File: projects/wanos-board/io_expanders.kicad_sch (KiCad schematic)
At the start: 17 parts, among them U1 PCA9554PW, U2 PCA9554PW

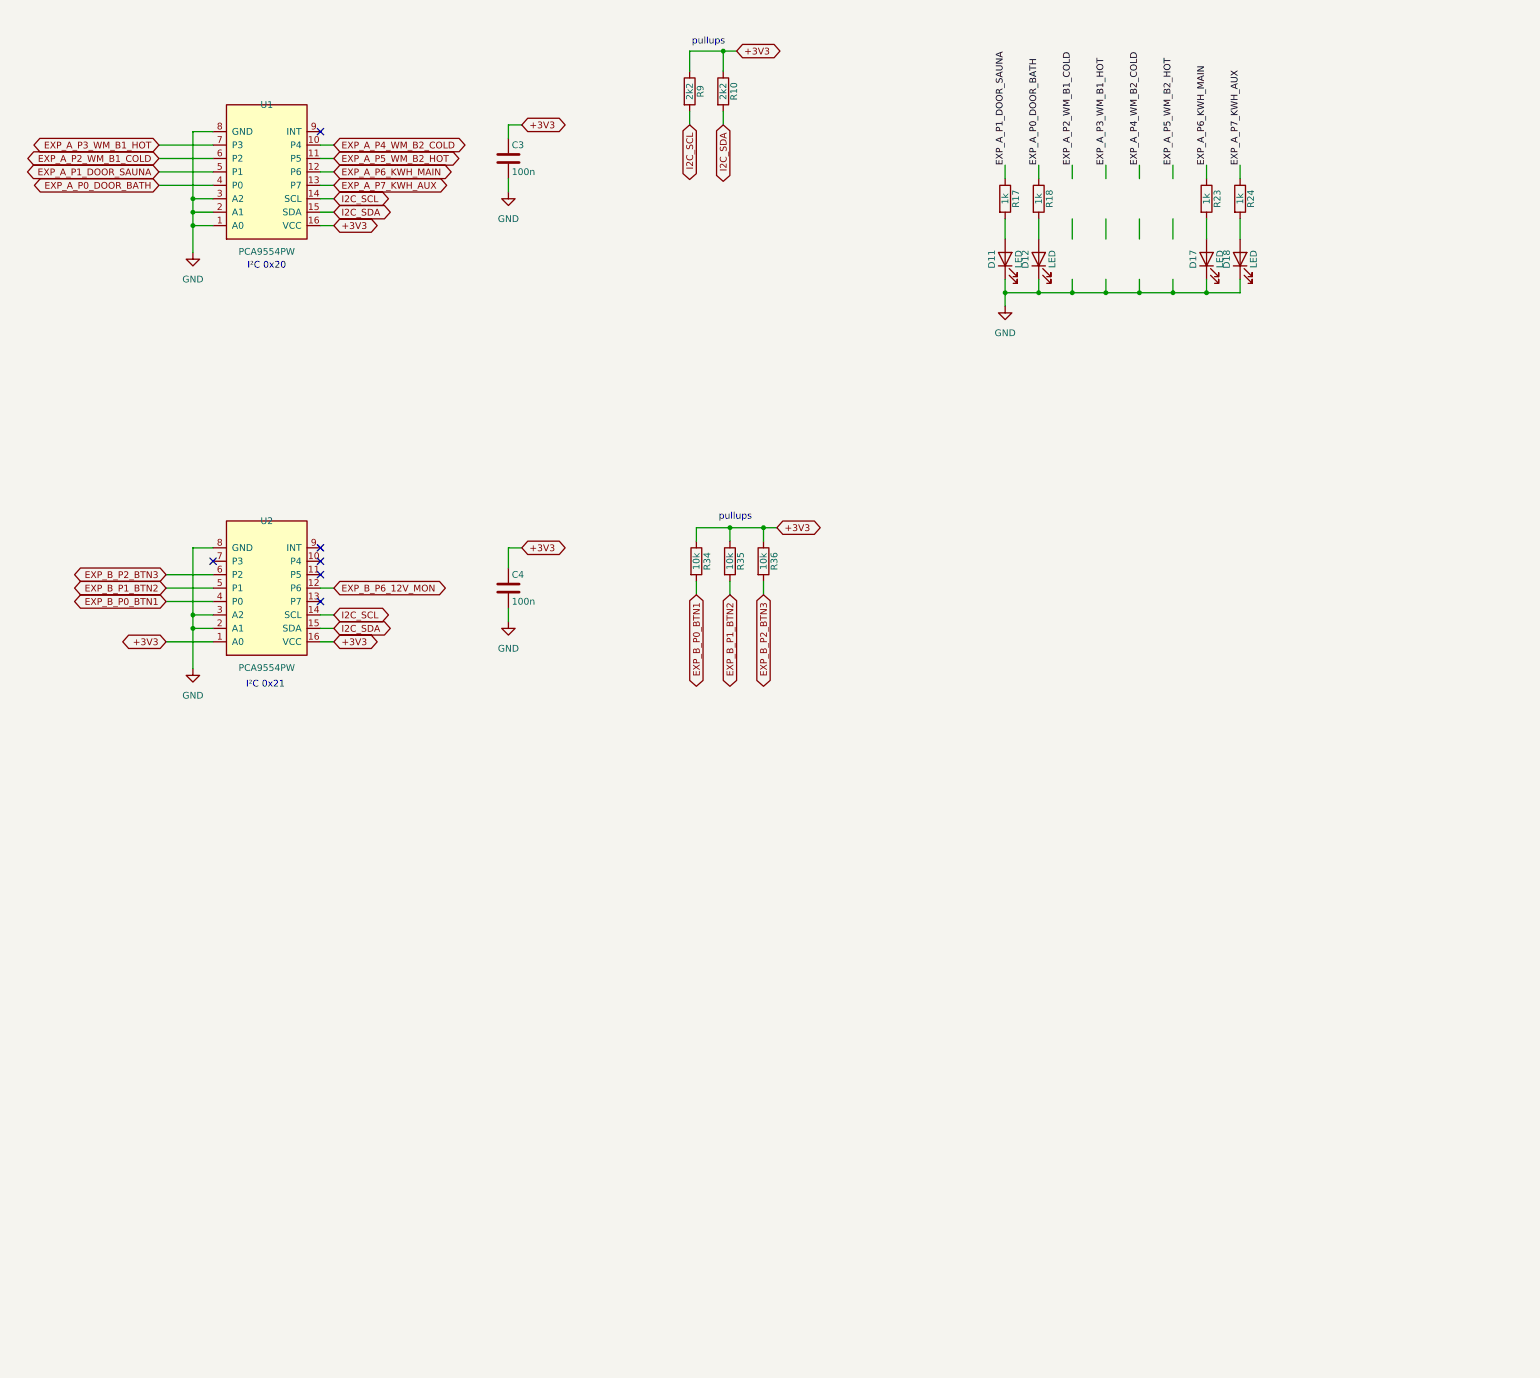
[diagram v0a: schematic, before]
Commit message: schema updates
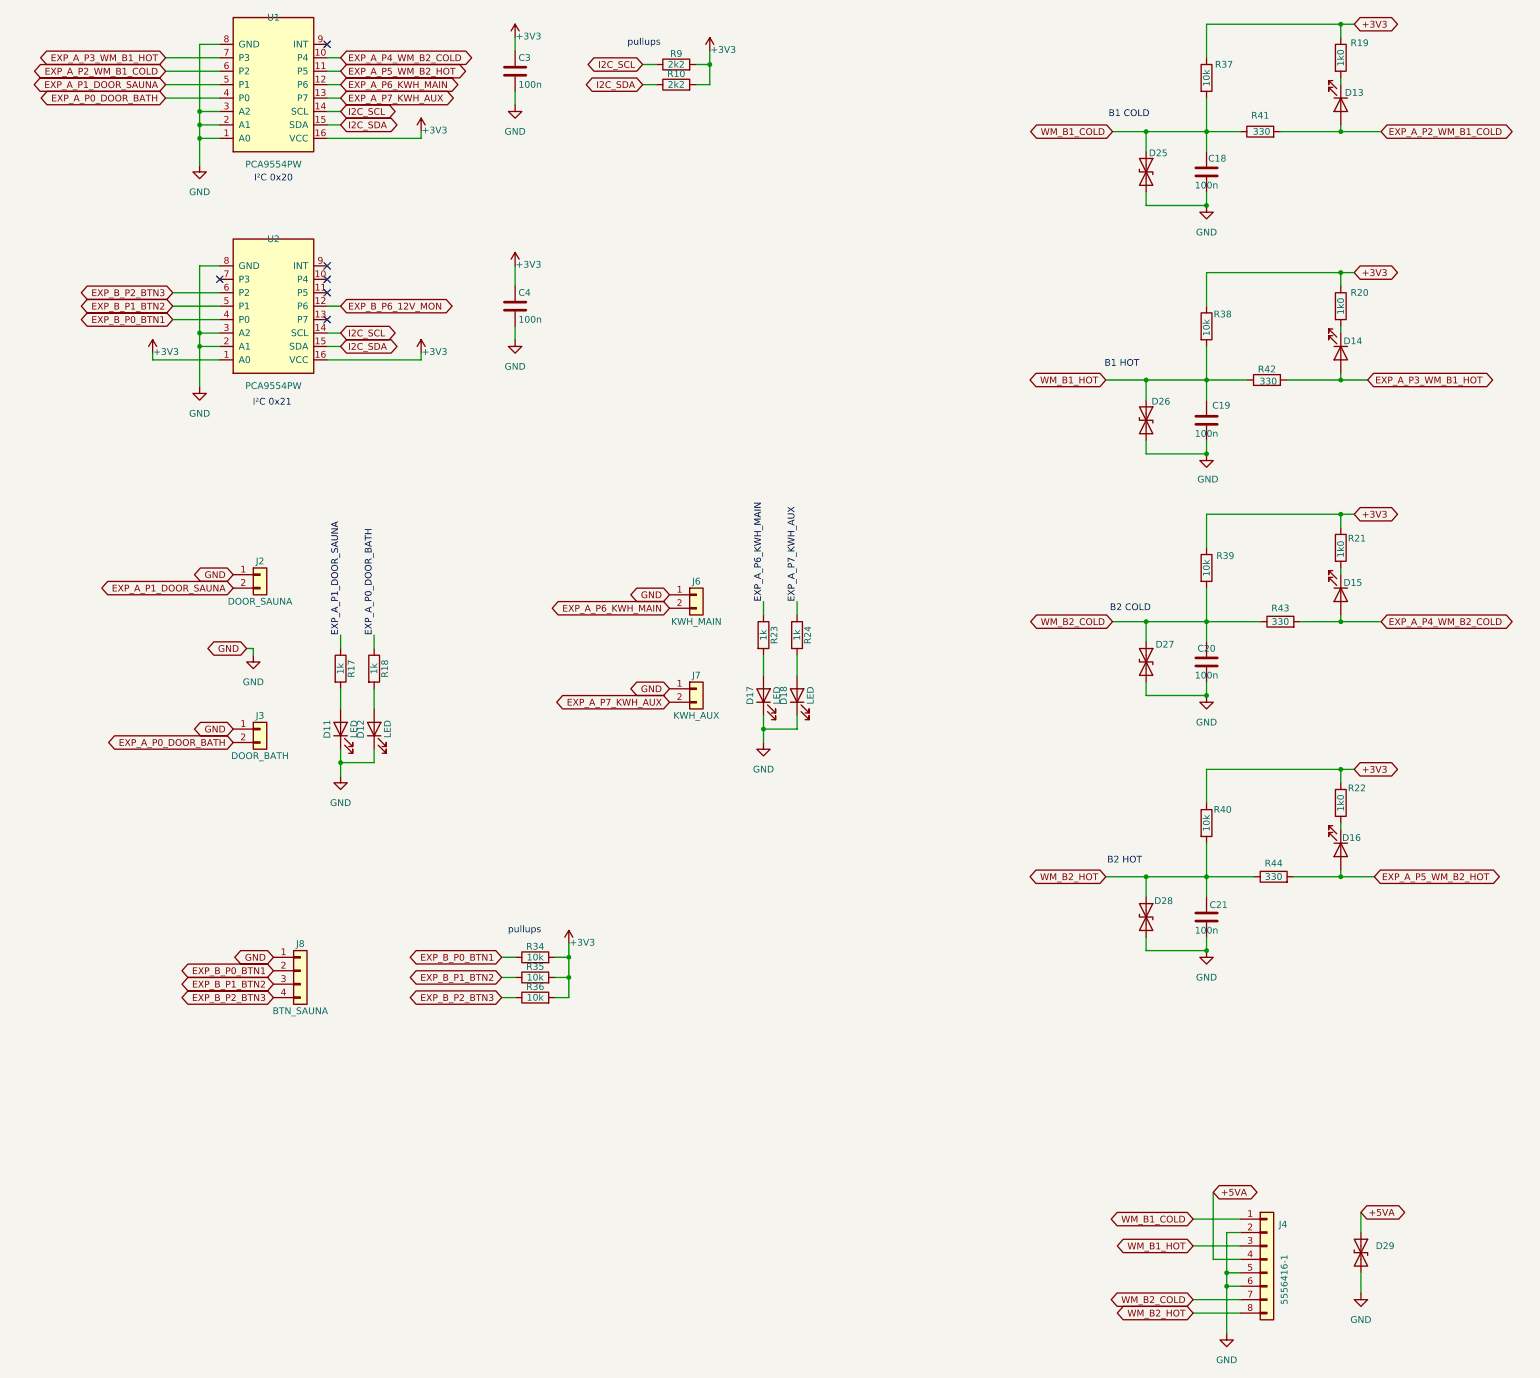
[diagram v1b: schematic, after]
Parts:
- added C18, C19, C20, C21: 100n, Capacitor_SMD:C_0805_2012Metric, symbol Device:C
- added D13, D14, D15, D16: LED, LED_SMD:LED_0805_2012Metric, symbol Device:LED
- added D25, D26, D27, D28: PESD5V0S1BA, Diode_SMD:D_SOD-323, symbol Device:D_TVS
- added D29: SMBJ5.0A, Diode_SMD:D_SMB, symbol Device:D_TVS
- added J2: DOOR_SAUNA, Connector_JST:JST_XH_B2B-XH-A_1x02_P2.50mm_Vertical, symbol Connector_Generic:Conn_01x02
- added J3: DOOR_BATH, Connector_JST:JST_XH_B2B-XH-A_1x02_P2.50mm_Vertical, symbol Connector_Generic:Conn_01x02
- added J4: 5556416-1, Connector_RJ:RJ45_Amphenol_54602-x08_Horizontal, symbol Connector_Generic:Conn_01x08
- added J6: KWH_MAIN, Connector_JST:JST_XH_B2B-XH-A_1x02_P2.50mm_Vertical, symbol Connector_Generic:Conn_01x02
- added J7: KWH_AUX, Connector_JST:JST_XH_B2B-XH-A_1x02_P2.50mm_Vertical, symbol Connector_Generic:Conn_01x02
- added J8: BTN_SAUNA, Connector_JST:JST_XH_B4B-XH-A_1x04_P2.50mm_Vertical, symbol Connector_Generic:Conn_01x04
- added R19, R20, R21, R22: 1k0, Resistor_SMD:R_0805_2012Metric, symbol Device:R
- added R37, R38, R39, R40: 10k, Resistor_SMD:R_0805_2012Metric, symbol Device:R
- added R41, R42, R43, R44: 330, Resistor_SMD:R_0805_2012Metric, symbol Device:R
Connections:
- net +3V3: now also R10.2, R34.2, R35.2, R36.2, R9.2, R19.1, R20.1, R21.1, R22.1, R37.1, R38.1, R39.1, R40.1; no longer R10.1, R34.1, R35.1, R36.1, R9.1
- net EXP_A_P0_DOOR_BATH: now also J3.2 (Pin_2)
- net EXP_A_P1_DOOR_SAUNA: now also J2.2 (Pin_2)
- net EXP_A_P2_WM_B1_COLD: now also D13.2 (A), R41.2
- net EXP_A_P3_WM_B1_HOT: now also D14.2 (A), R42.2
- net EXP_A_P4_WM_B2_COLD: now also D15.2 (A), R43.2
- net EXP_A_P5_WM_B2_HOT: now also D16.2 (A), R44.2
- net EXP_A_P6_KWH_MAIN: now also J6.2 (Pin_2)
- net EXP_A_P7_KWH_AUX: now also J7.2 (Pin_2)
- net EXP_B_P0_BTN1: now also R34.1, J8.2 (Pin_2); no longer R34.2
- net EXP_B_P1_BTN2: now also R35.1, J8.3 (Pin_3); no longer R35.2
- net EXP_B_P2_BTN3: now also R36.1, J8.4 (Pin_4); no longer R36.2
- net GND: now also C18.2, C19.2, C20.2, C21.2, D25.2 (A2), D26.2 (A2), D27.2 (A2), D28.2 (A2), D29.2 (A2), J2.1 (Pin_1), J3.1 (Pin_1), J4.2 (Pin_2), J4.5 (Pin_5), J4.6 (Pin_6), J6.1 (Pin_1), J7.1 (Pin_1), J8.1 (Pin_1)
- net I2C_SCL: now also R9.1; no longer R9.2
- net I2C_SDA: now also R10.1; no longer R10.2
- new net: D16.1 (K), R22.2
- new net: D14.1 (K), R20.2
- new net: D13.1 (K), R19.2
- new net: D15.1 (K), R21.2
- new net +5VA: D29.1 (A1), J4.4 (Pin_4)
- new net WM_B1_COLD: C18.1, D25.1 (A1), J4.1 (Pin_1), R37.2, R41.1
- new net WM_B1_HOT: C19.1, D26.1 (A1), J4.3 (Pin_3), R38.2, R42.1
- new net WM_B2_COLD: C20.1, D27.1 (A1), J4.7 (Pin_7), R39.2, R43.1
- new net WM_B2_HOT: C21.1, D28.1 (A1), J4.8 (Pin_8), R40.2, R44.1
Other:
- note added: "B1 COLD"
- note added: "B1 HOT"
- note added: "B2 COLD"
- note added: "B2 HOT"
- title: (none) -> wanos-pcb-v1 IO Expanders
